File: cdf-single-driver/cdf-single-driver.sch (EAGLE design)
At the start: 30 parts, among them IC1 R-789.0-0.5, IC2 UCC27423

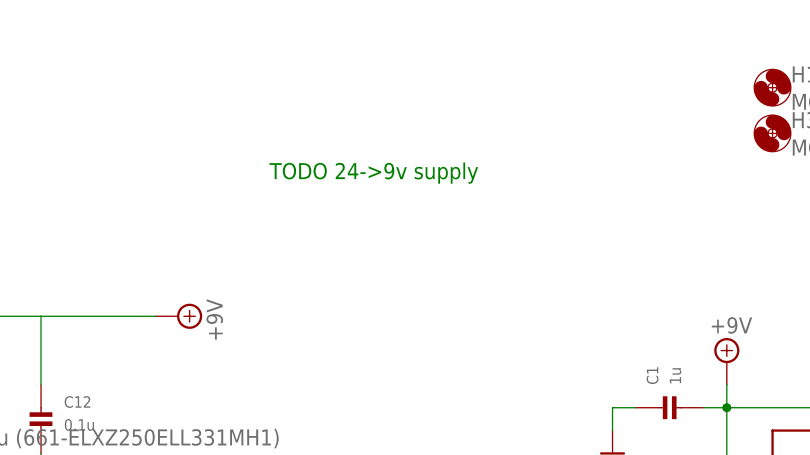
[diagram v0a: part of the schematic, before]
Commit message: cdf-single-driver wip
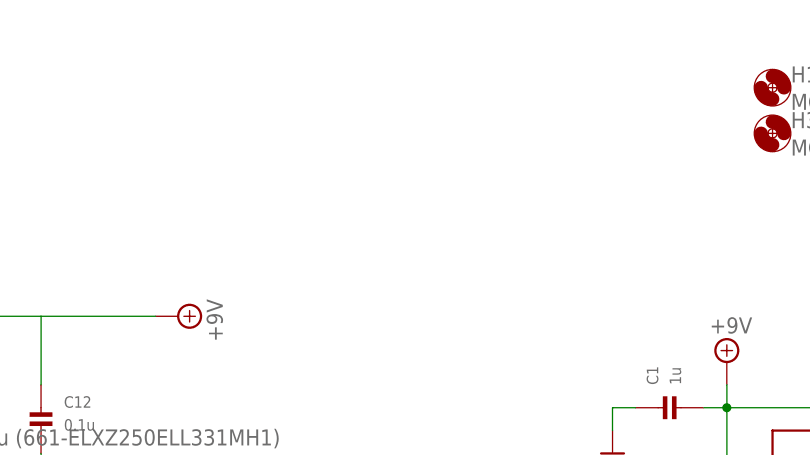
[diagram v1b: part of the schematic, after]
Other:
- note removed: "TODO 24->9v supply"
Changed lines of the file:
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@@
 <part name="H4" library="holes" deviceset="MOUNT-HOLE" device="3.3"/>
 <part name="24V" library="con-ptr500" deviceset="AK500/2" device=""/>
-<part name="P+3" library="supply1" deviceset="+24V" device=""/>
-<part name="GND8" library="microbuilder" deviceset="GND" device=""/>
 <part name="IC1" library="r-78xx_10" deviceset="R-78*-0.5" device="" technology="9.0"/>
 <part name="C8" library="rcl" deviceset="CPOL-US" device="E3.5-8" value="220u"/>
@@
 <part name="SUPPLY2" library="supply2" deviceset="+9V" device=""/>
 <part name="D3" library="diode" deviceset="DIODE-" device="SOD123"/>
+<part name="P+3" library="supply1" deviceset="+24V" device=""/>
+<part name="GND8" library="microbuilder" deviceset="GND" device=""/>
 </parts>
 <sheets>
 <sheet>
 <plain>
-<text x="0" y="88.9" size="1.778" layer="91">TODO 24-&gt;9v supply</text>
 </plain>
 <instances>
@@
 <instance part="24V" gate="-1" x="-45.72" y="101.6"/>
 <instance part="24V" gate="-2" x="-45.72" y="96.52"/>
-<instance part="P+3" gate="1" x="-33.02" y="101.6" rot="R270"/>
-<instance part="GND8" gate="G$1" x="-33.02" y="96.52" rot="R90"/>
 <instance part="IC1" gate="G$1" x="-55.88" y="73.66"/>
 <instance part="C8" gate="G$1" x="-86.36" y="68.58"/>
@@
 <instance part="SUPPLY2" gate="G$1" x="-10.16" y="73.66" rot="R270"/>
 <instance part="D3" gate="G$1" x="-55.88" y="83.82" rot="R180"/>
+<instance part="P+3" gate="1" x="-33.02" y="101.6" rot="R270"/>
+<instance part="GND8" gate="G$1" x="-33.02" y="96.52" rot="R90"/>
 </instances>
 <busses>
@@
 <pinref part="GND7" gate="G$1" pin="GND"/>
 <wire x1="162.56" y1="40.64" x2="160.02" y2="40.64" width="0.1524" layer="91"/>
-</segment>
-<segment>
-<pinref part="24V" gate="-2" pin="KL"/>
-<pinref part="GND8" gate="G$1" pin="GND"/>
-<wire x1="-35.56" y1="96.52" x2="-40.64" y2="96.52" width="0.1524" layer="91"/>
 </segment>
 <segment>
@@
 <wire x1="-35.56" y1="58.42" x2="-35.56" y2="53.34" width="0.1524" layer="91"/>
 </segment>
+<segment>
+<pinref part="24V" gate="-2" pin="KL"/>
+<wire x1="-35.56" y1="96.52" x2="-40.64" y2="96.52" width="0.1524" layer="91"/>
+<pinref part="GND8" gate="G$1" pin="GND"/>
+</segment>
 </net>
 <net name="N$1" class="0">
@@
 <wire x1="116.84" y1="40.64" x2="116.84" y2="35.56" width="0.1524" layer="91"/>
 <junction x="127" y="40.64"/>
-</segment>
-<segment>
-<pinref part="24V" gate="-1" pin="KL"/>
-<pinref part="P+3" gate="1" pin="+24V"/>
-<wire x1="-35.56" y1="101.6" x2="-40.64" y2="101.6" width="0.1524" layer="91"/>
 </segment>
 <segment>
@@
 <wire x1="-68.58" y1="83.82" x2="-68.58" y2="73.66" width="0.1524" layer="91"/>
 </segment>
-</net>
+<segment>
+<pinref part="24V" gate="-1" pin="KL"/>
+<wire x1="-35.56" y1="101.6" x2="-40.64" y2="101.6" width="0.1524" layer="91"/>
+<pinref part="P+3" gate="1" pin="+24V"/>
+</segment>
+</net>
